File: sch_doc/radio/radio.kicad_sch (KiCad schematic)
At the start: 82 parts, among them J1 tun, J2 out, J8 vcc, J9 gnd, U1 ATTINY13A-PU, U2 TDA7088, U3 74HC595

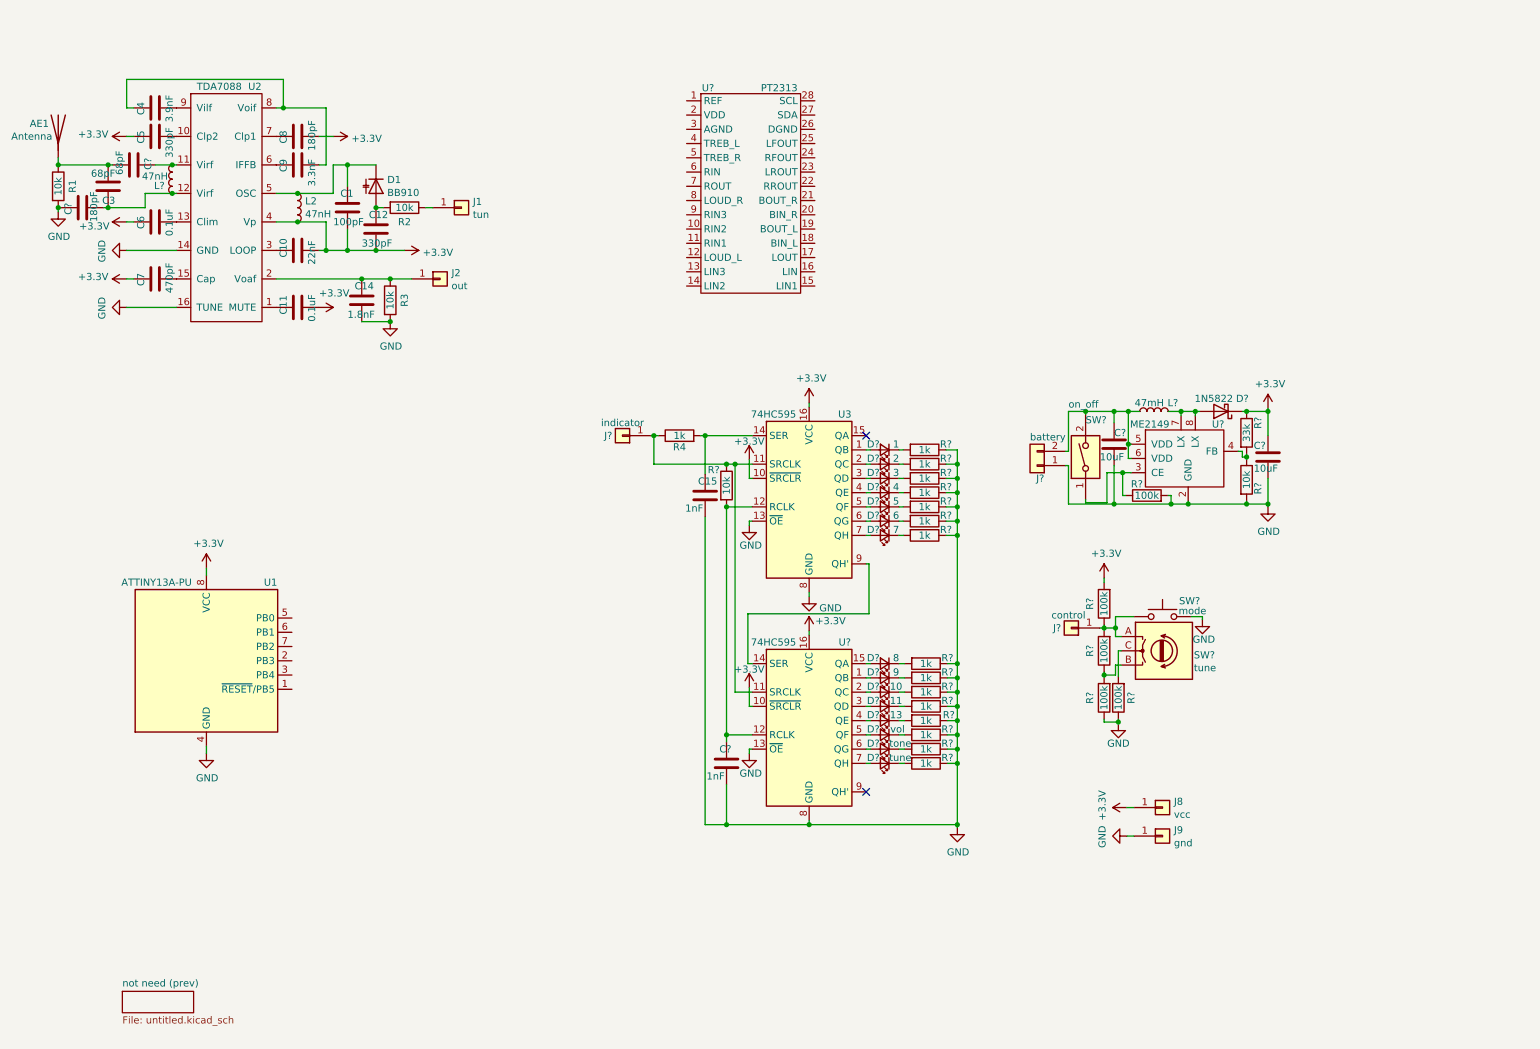
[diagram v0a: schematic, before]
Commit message: new schematics, I hope that it will be final
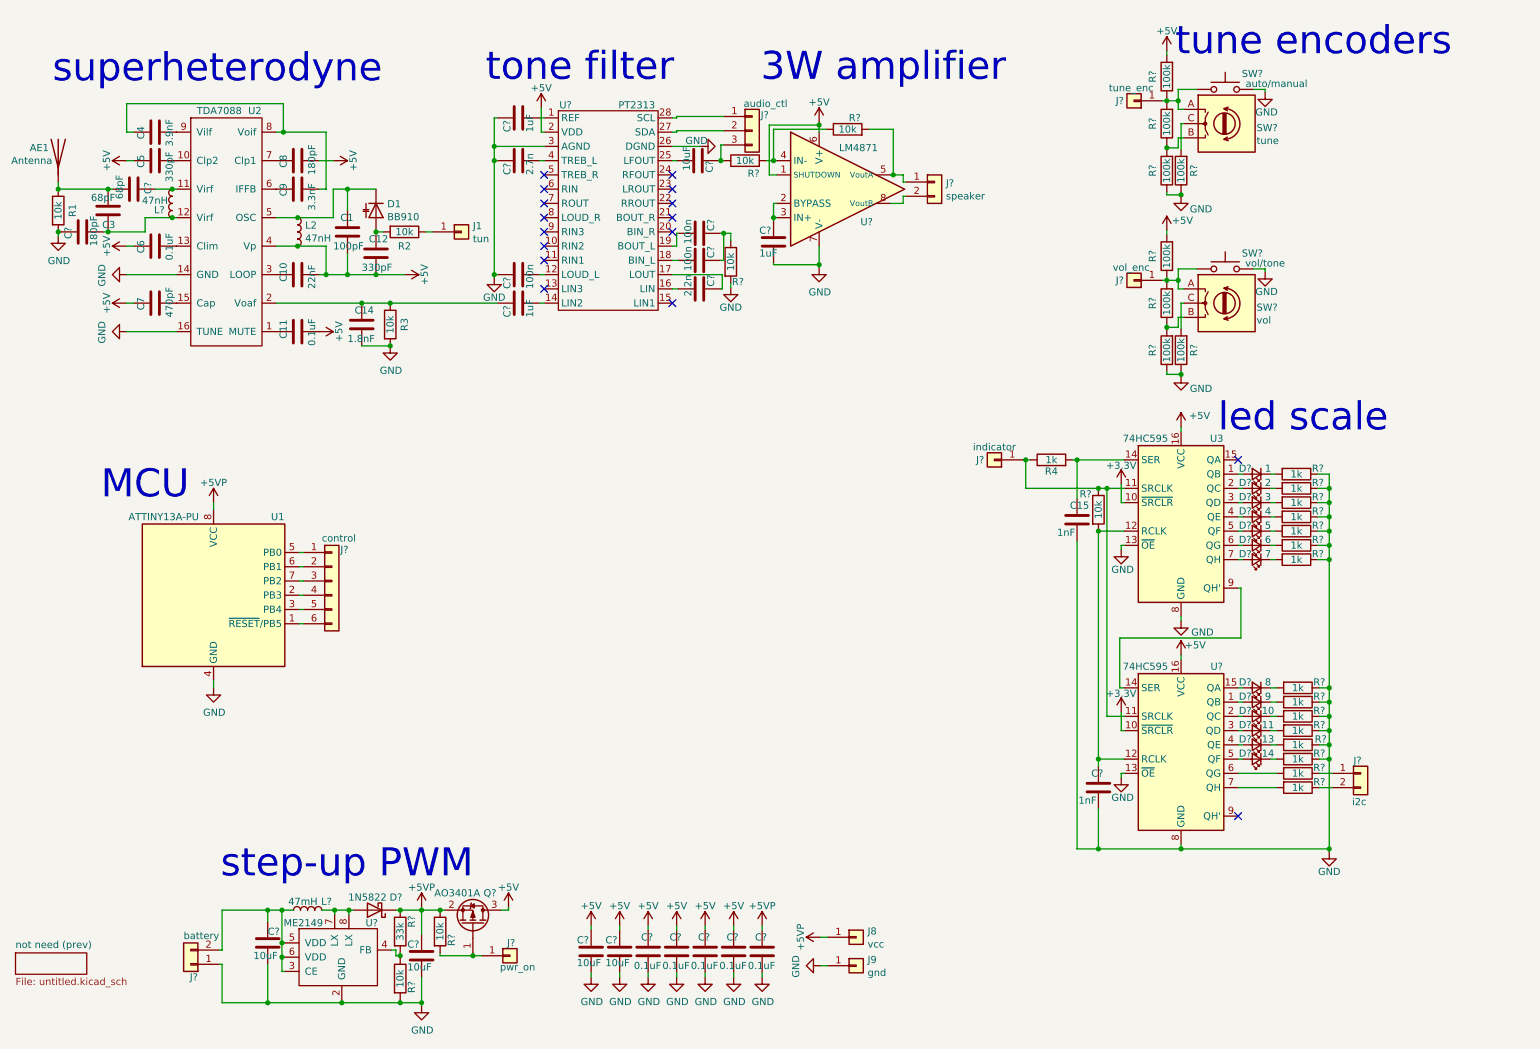
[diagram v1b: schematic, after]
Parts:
- removed D?: tune, symbol Device:LED_Small
- removed D?: tone, symbol Device:LED_Small
- removed D?: vol, symbol Device:LED_Small
- removed J2: out, Connector_Wire:SolderWirePad_1x01_SMD_5x10mm, symbol Connector_Generic:Conn_01x01
- removed R?: 100k, symbol Device:R
- removed SW?: on_off, symbol Switch:SW_DIP_x01
- added C? (x3): 1uF, symbol Device:C
- added C? (x5): 0.1uF, Capacitor_SMD:C_0603_1608Metric, symbol Device:C
- added C? (x3): 100n, symbol Device:C
- added C?: 2.7n, symbol Device:C
- added C? (x3): 10uF, symbol Device:C
- added C?: 2.2n, symbol Device:C
- added D?: 14, symbol Device:LED_Small
- added J?: tune_enc, Connector_Wire:SolderWirePad_1x01_SMD_5x10mm, symbol Connector_Generic:Conn_01x01
- added J?: i2c, symbol Connector_Generic:Conn_01x02
- added J?: audio_ctl, symbol Connector_Generic:Conn_01x03
- added J?: pwr_on, Connector_Wire:SolderWirePad_1x01_SMD_5x10mm, symbol Connector_Generic:Conn_01x01
- added J?: control, symbol Connector_Generic:Conn_01x06
- added J?: speaker, symbol Connector_Generic:Conn_01x02
- added Q?: AO3401A, Package_TO_SOT_SMD:SOT-23, symbol Transistor_FET:AO3401A
- added R? (x4): 100k, Resistor_SMD:R_0805_2012Metric, symbol Device:R
- added R? (x4): 10k, symbol Device:R
- added SW?: tune, symbol Device:RotaryEncoder
- added SW?: auto/manual, symbol Switch:SW_Push
- added U?: LM4871, Package_SO:SOIC-8_3.9x4.9mm_P1.27mm, symbol local:LM4871
- J?: value control -> vol_enc
- SW?: value mode -> vol/tone
- SW?: value tune -> vol
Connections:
- net +3.3V: no longer C1.1, C10.1, C11.1, C12.1, C5.2, C6.2, C7.2, C8.1, C?.2, D?.1 (K), J8.1 (Pin_1), L2.2, R?.1, R?.2, U1.8 (VCC), U2.4 (Vp), U3.16 (VCC), U?.16 (VCC)
- net GND: now also U?.26 (DGND), U?.3 (AGND), C?.1, C?.1, C?.1, C?.1, C?.1, C?.1, C?.1, C?.1, C?.2, C?.2, C?.2, R?.1, R?.1, R?.2, SW?.2, U?.7 (V-); no longer R?.1, R?.1
- net at U1.1 (~{RESET}/PB5): now also J?.6 (Pin_6)
- net at U1.2 (PB3): now also J?.4 (Pin_4)
- net at U1.3 (PB4): now also J?.5 (Pin_5)
- net at U1.5 (PB0): now also J?.1 (Pin_1)
- net at U1.6 (PB1): now also J?.2 (Pin_2)
- net at U1.7 (PB2): now also J?.3 (Pin_3)
- net at C14.2, R3.1, U2.2 (Voaf): now also C?.2
- net at C?.2, J?.2 (Pin_2), L?.1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: now also U?.3 (CE)
- net at R?.2: now also U?.6 (QG)
- net at R?.2: now also U?.7 (QH)
- net at U?.1 (REF): now also C?.1
- net at U?.12 (LOUD_L): now also C?.1
- net at U?.14 (LIN2): now also C?.1
- net at U?.16 (LIN): now also C?.1
- net at U?.17 (LOUT): now also C?.2
- net at U?.18 (BIN_L): now also C?.1
- net at U?.19 (BOUT_L): now also C?.1
- net +5V: now reaches U?.2 (VDD)
- net +5V: now also C1.1, C10.1, C11.1, C12.1, C5.2, C6.2, C7.2, C8.1, L2.2, R?.2, U2.4 (Vp), U3.16 (VCC), U?.16 (VCC), C?.2, C?.2, C?.2, C?.2, C?.2, C?.2, Q?.3 (D), R?.2, U?.1 (SHUTDOWN), U?.6 (V+)
- net at U?.25 (LFOUT): now also C?.1
- net at U?.27 (SDA): now also J?.2 (Pin_2)
- net at U?.28 (SCL): now also J?.1 (Pin_1)
- net at U?.4 (TREB_L): now also C?.1
- net at U?.5 (QF): now also D?.2 (A)
- net at R?.2: now also D?.1 (K)
- new net: J?.1 (Pin_1), R?.1
- new net: J?.2 (Pin_2), R?.1
- new net: C?.2, U?.2 (BYPASS), U?.3 (IN+)
- new net: J?.1 (Pin_1), R?.1, R?.2, SW?.1, SW?.A
- new net: R?.1, R?.2, SW?.B
- new net: R?.2, SW?.C
- new net: R?.1, R?.2, U?.4 (IN-)
- new net: J?.1 (Pin_1), R?.2, U?.5 (VoutA)
- new net: C?.2, J?.3 (Pin_3), R?.1
- new net: J?.1 (Pin_1), Q?.1 (G), R?.2
- new net: J?.2 (Pin_2), U?.8 (VoutB)
- new net: C?.2, C?.2, R?.1
- new net +5VP: C?.2, C?.2, D?.1 (K), J8.1 (Pin_1), Q?.2 (S), R?.1, R?.1, U1.8 (VCC)
- no-connect marks 2 -> 16
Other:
- note added: "3W amplifier"
- note added: "MCU"
- note added: "led scale"
- note added: "step-up PWM"
- note added: "superheterodyne"
- note added: "tone filter"
- note added: "tune encoders"
- moved on the sheet: AE1, C1, C10, C11, C12, C14, C15, C3, C4, C5, C6, C7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
